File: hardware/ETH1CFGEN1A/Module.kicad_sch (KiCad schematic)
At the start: 3 parts, among them J601 Conn_02x04_Odd_Even, J602 Conn_02x04_Odd_Even, J603 Conn_Coaxial

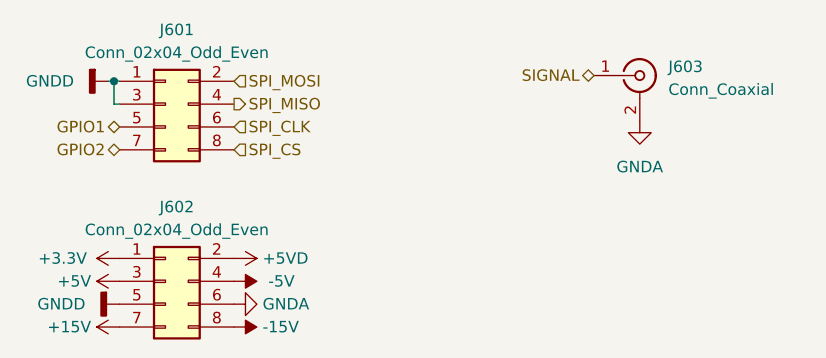
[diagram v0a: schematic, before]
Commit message: Development
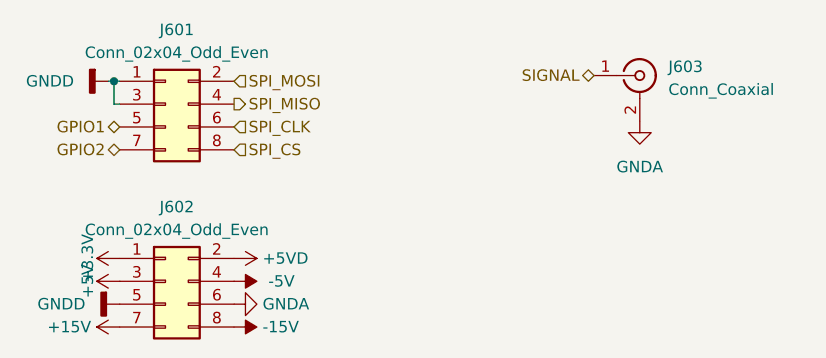
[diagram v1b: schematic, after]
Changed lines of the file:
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@@
       (effects (font (size 1.27 1.27)) hide)
     )
-    (property "Value" "+3.3V" (at 118.745 86.995 90)
+    (property "Value" "+3.3V" (at 121.539 86.995 0)
       (effects (font (size 1.27 1.27)))
     )
@@
       (effects (font (size 1.27 1.27)) hide)
     )
-    (property "Value" "+5V" (at 121.92 89.535 90)
-      (effects (font (size 1.27 1.27)) (justify left))
+    (property "Value" "+5V" (at 121.539 89.535 0)
+      (effects (font (size 1.27 1.27)))
     )
     (property "Footprint" "" (at 125.095 89.535 0)

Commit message: Development
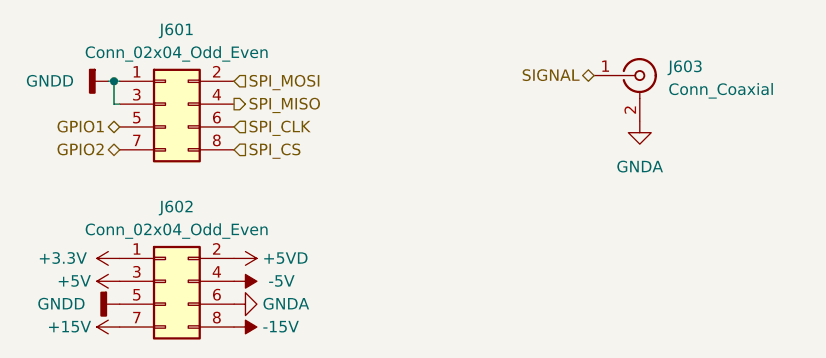
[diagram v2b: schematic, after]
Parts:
- J601, J602: footprint (none) -> Connector_PinHeader_2.54mm:PinHeader_2x04_P2.54mm_Vertical
- J603: footprint (none) -> ETH1CFGEN1:NX5032GA
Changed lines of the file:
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@@
       (effects (font (size 1.27 1.27)))
     )
-    (property "Footprint" "" (at 130.175 69.85 0)
+    (property "Footprint" "Connector_PinHeader_2.54mm:PinHeader_2x04_P2.54mm_Vertical" (at 130.175 69.85 0)
       (effects (font (size 1.27 1.27)) hide)
     )
@@
       (effects (font (size 1.27 1.27)))
     )
-    (property "Footprint" "" (at 130.175 89.535 0)
+    (property "Footprint" "Connector_PinHeader_2.54mm:PinHeader_2x04_P2.54mm_Vertical" (at 130.175 89.535 0)
       (effects (font (size 1.27 1.27)) hide)
     )
@@
       (effects (font (size 1.27 1.27)) hide)
     )
-    (property "Value" "+3.3V" (at 121.539 86.995 0)
+    (property "Value" "+3.3V" (at 118.745 86.995 90)
       (effects (font (size 1.27 1.27)))
     )
@@
   )
   (symbol (lib_id "power:+5V") (at 125.095 89.535 90) (unit 1)
-    (in_bom yes) (on_board yes) (dnp no) (fields_autoplaced)
+    (in_bom yes) (on_board yes) (dnp no)
     (property "Reference" "#PWR0731" (at 128.905 89.535 0)
       (effects (font (size 1.27 1.27)) hide)
     )
-    (property "Value" "+5V" (at 121.539 89.535 0)
+    (property "Value" "+5V" (at 120.015 89.535 90)
       (effects (font (size 1.27 1.27)))
     )
@@
       (effects (font (size 1.27 1.27)) (justify left))
     )
-    (property "Footprint" "" (at 182.88 66.675 0)
-      (effects (font (size 1.27 1.27)) hide)
-    )
+    (property "Footprint" "ETH1CFGEN1:NX5032GA" (at 182.88 66.675 0)
+      (effects (font (size 1.27 1.27)) hide)
+    )
